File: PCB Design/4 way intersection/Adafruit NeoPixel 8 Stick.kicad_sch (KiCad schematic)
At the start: 13 parts, among them CN1 1X4SMT, CN2 1X4SMT, CN3 1X4SMT, CN4 1X4SMT

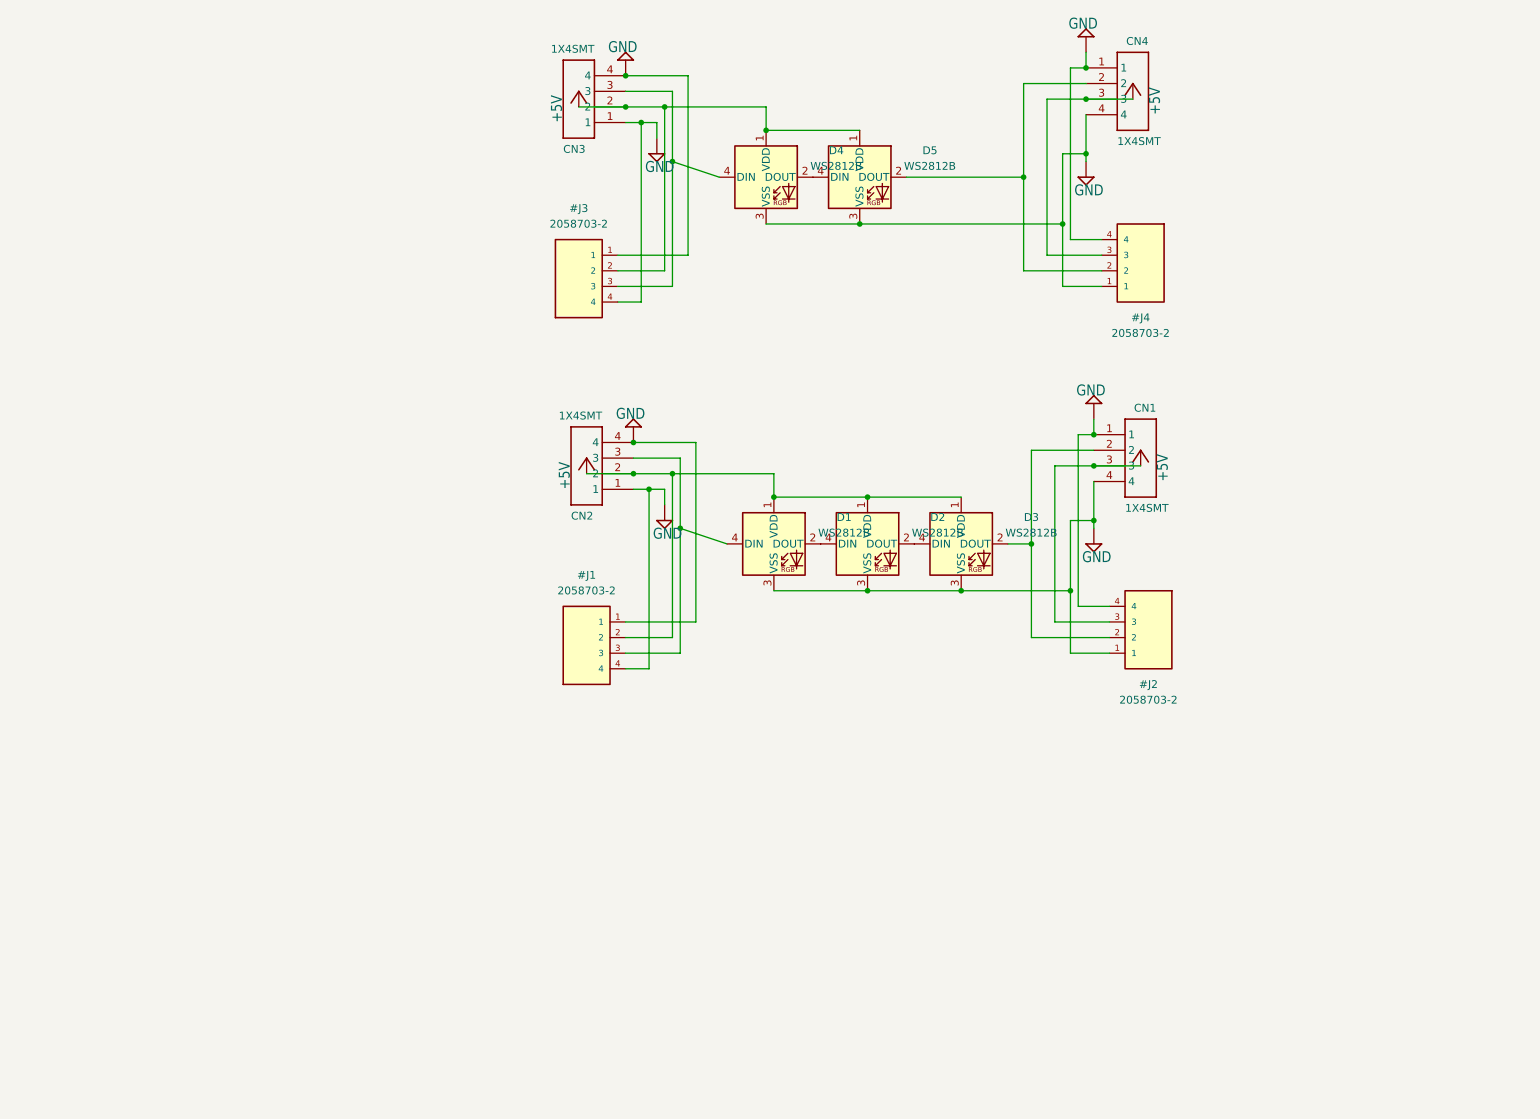
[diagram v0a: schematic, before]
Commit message: 6 pin
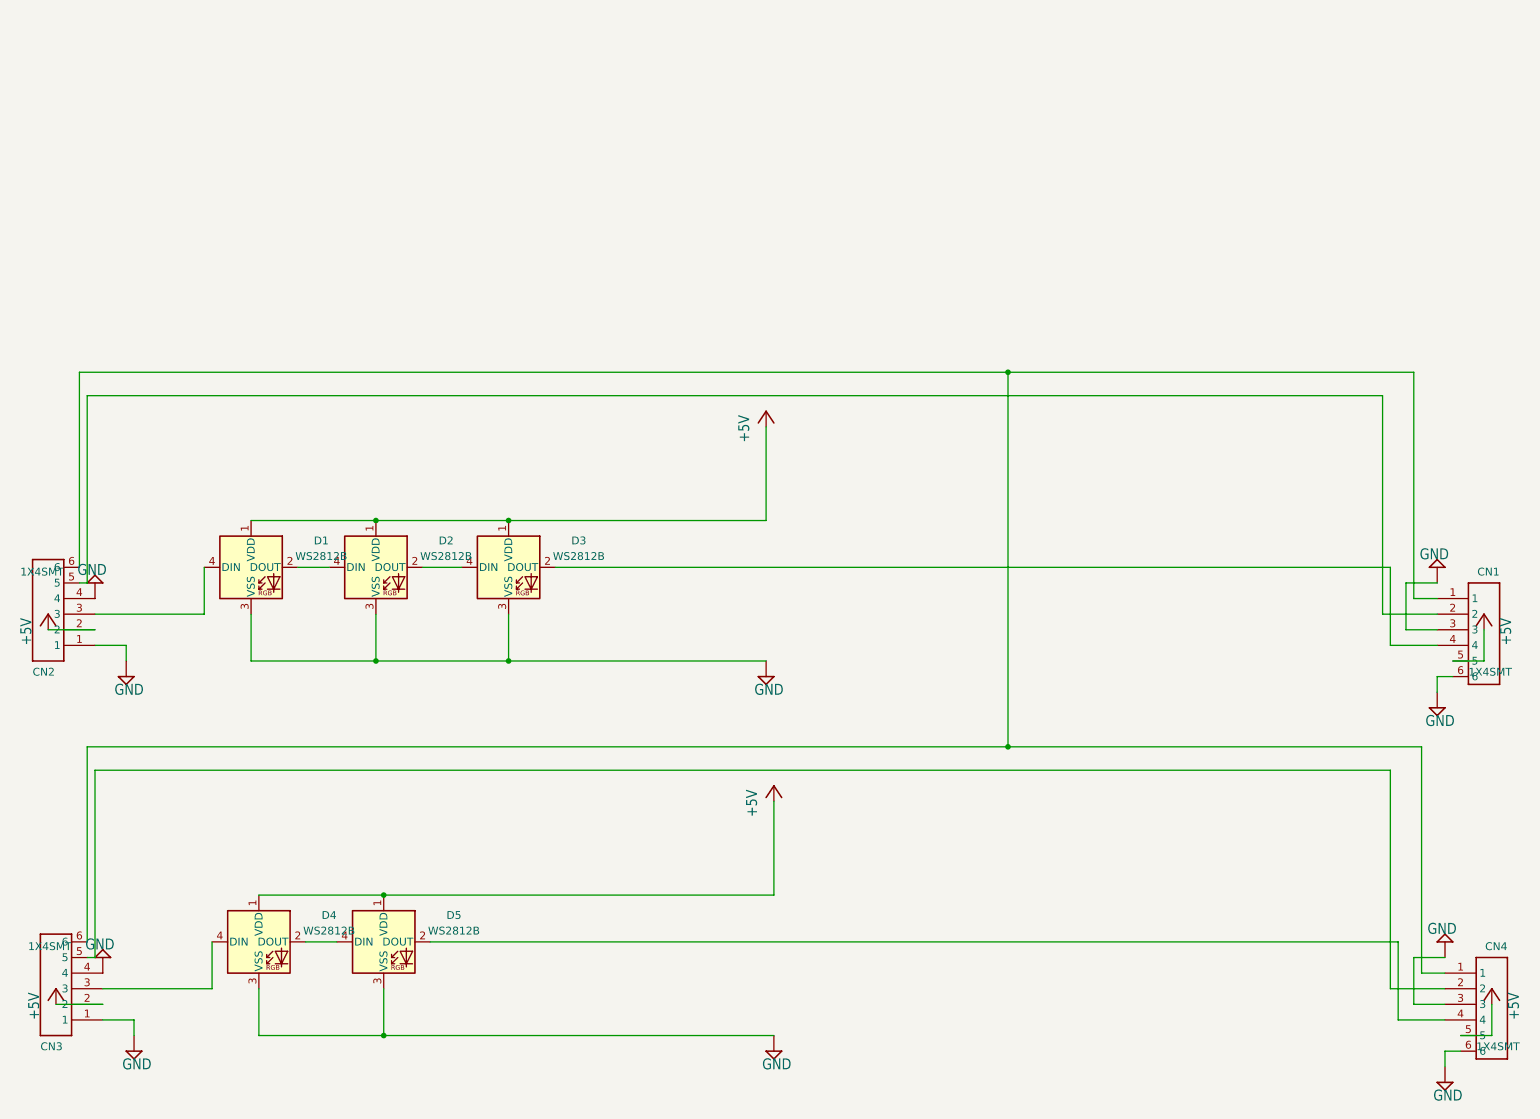
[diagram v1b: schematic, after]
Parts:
- removed #J1, #J2, #J3, #J4: 2058703-2, TE_2058703-2, symbol 2058703-2:2058703-2
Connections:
- net +5V: now also CN1.5, CN4.5; no longer CN1.3, CN4.3
- net GND: now also CN1.3, CN1.6, CN4.3, CN4.6; no longer CN1.1, CN1.4, CN4.1, CN4.4
- net at D3.2 (DOUT): now also CN1.4; no longer CN1.2
- net at D5.2 (DOUT): now also CN4.4; no longer CN4.2
- new net: CN1.2, CN2.5
- new net: CN1.1, CN2.6, CN3.6, CN4.1
- new net: CN3.5, CN4.2
